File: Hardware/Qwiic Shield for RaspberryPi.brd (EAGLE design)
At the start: 52.3 x 23 mm, 22 parts, among them J1 Qwiic Right Angle, J6 Qwiic Right Angle, J7 Qwiic Right Angle, J8 Qwiic Right Angle, U2 3.3V/600mA

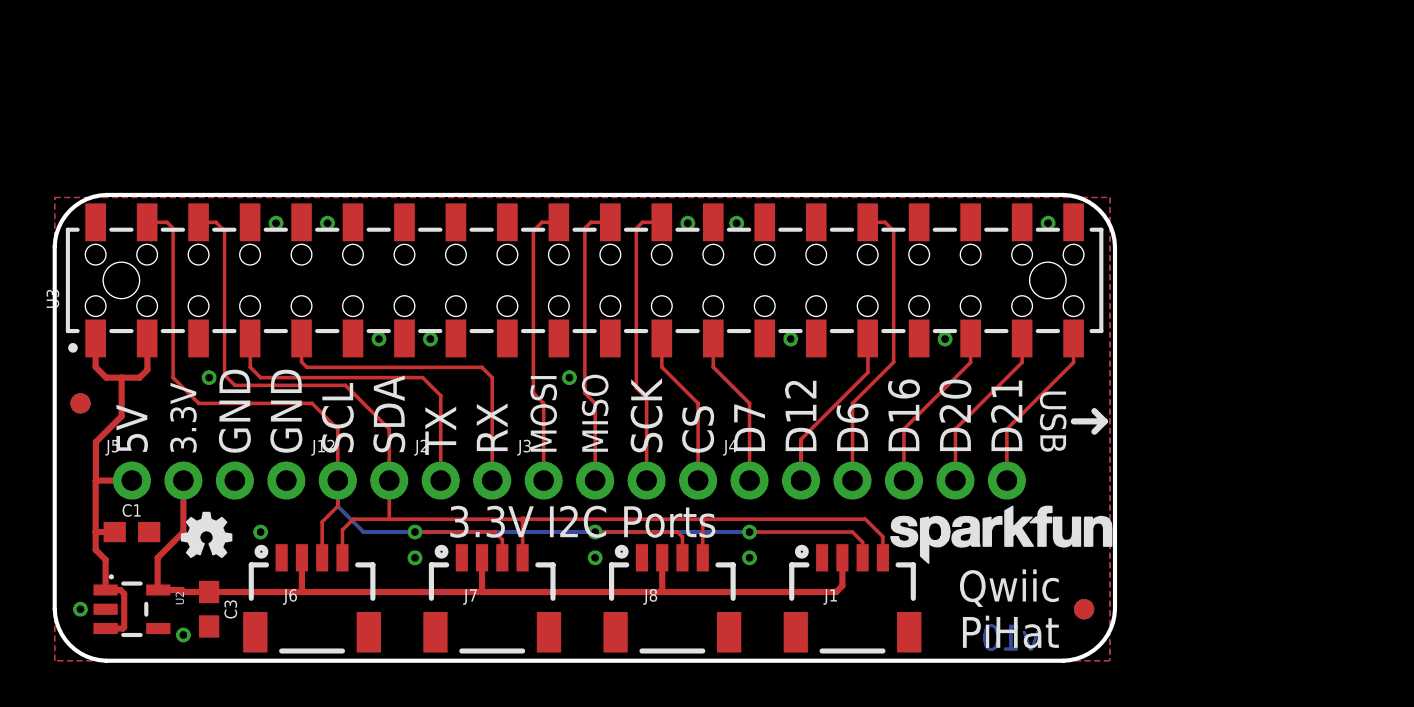
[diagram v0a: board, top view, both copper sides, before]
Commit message: v20 Initial Commit
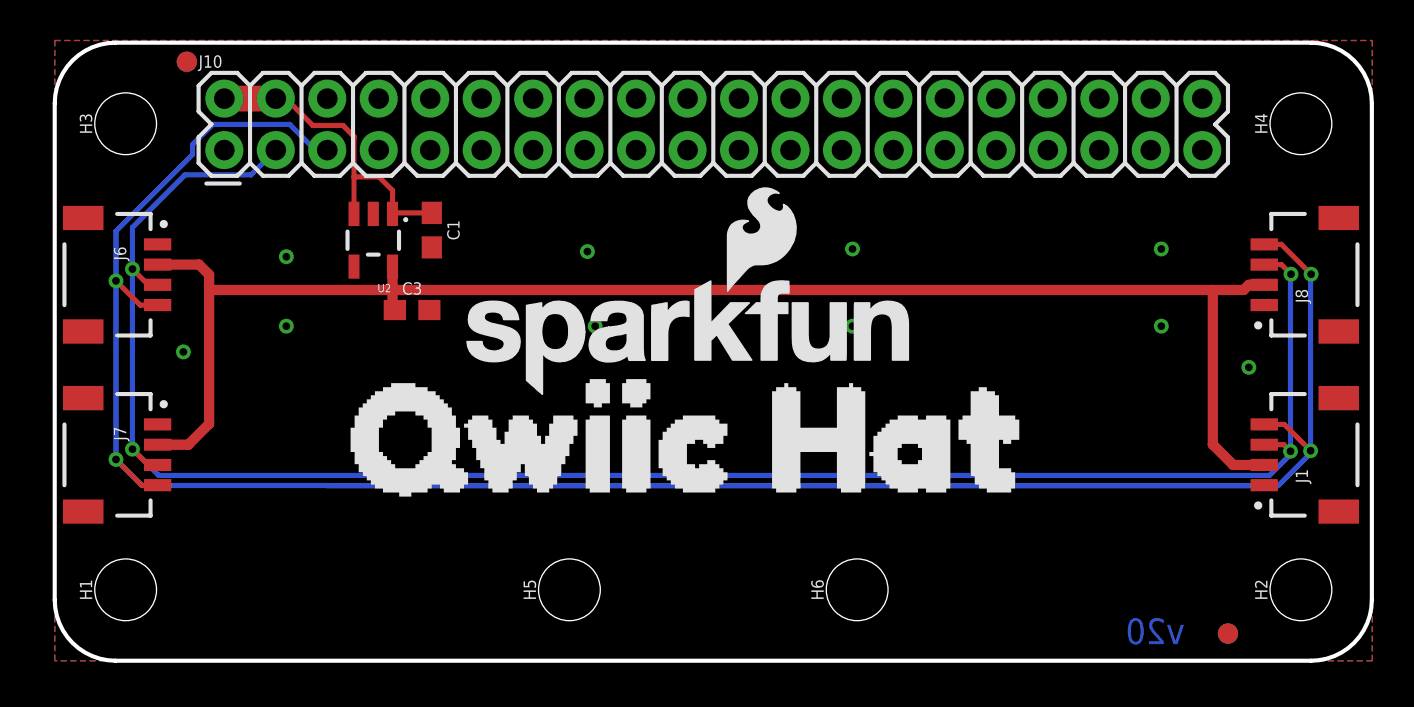
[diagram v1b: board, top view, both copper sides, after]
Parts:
- removed J12, J2: (no value), SparkFun-Connectors:1X02_NO_SILK
- removed J3, J5: (no value), SparkFun-Connectors:1X04_NO_SILK
- removed J4: (no value), SparkFun-Connectors:1X06_NO_SILK
- removed LOGO1: OSHW-LOGOMINI, SparkFun-Aesthetics:OSHW-LOGO-MINI
- removed U$2: SFE_LOGO_NAME.1_INCH, SparkFun-Aesthetics:SFE_LOGO_NAME_.1
- removed U3: (no value), SparkFun-Connectors:RASPBERRY_PI_SHIELD_BOTTOM_ENTRY_NOHOLES
- added H1, H2, H3, H4, H5, H6: STAND-OFFTIGHT, SparkFun-Hardware:STAND-OFF-TIGHT
- added J10: RASPBERRYPI-40-PIN-GPIO_PTH_NO_SHROUD, SparkFun-Connectors:2X20
- added LOGO3: SFE_LOGO_NAME_FLAME.2_INCH, SparkFun-Aesthetics:SFE_LOGO_NAME_FLAME_.2
- J1, J6, J7, J8: device SparkFun-Connectors:1X04_1MM_RA -> SparkFun-Connectors:JST04_1MM_RA
- U$1: value SFE_LOGO_FLAME.1_INCH -> (none); device SparkFun-Aesthetics:SFE_LOGO_FLAME_.1 -> Qwiic Hat:QWIIC_HAT0
- moved J8 32.4 mm to (59.7, 19.1), turned to 90 degrees
- moved U2 21.8 mm to (15.7, 20.8), turned to 180 degrees
- moved C1 21.0 mm to (18.6, 21.2), turned to 270 degrees
- moved J1 20.9 mm to (59.7, 10.2), turned to 90 degrees
- moved C3 17.8 mm to (17.6, 17.3), turned to 0 degrees
- moved FD1 17.7 mm to (6.52, 29.6)
- moved FD4 17.7 mm to (6.52, 29.6)
- moved J7 17.3 mm to (5.08, 10.2), turned to 270 degrees
- moved J6 15.9 mm to (5.08, 19.1), turned to 270 degrees
- moved U$1 8.05 mm to (10.0, 11.0), flipped to the top
- moved FD2 7.20 mm to (57.9, 1.34)
- moved FD3 7.20 mm to (57.9, 1.34)
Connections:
- removed net CS: J3.4, U3.24
- removed net D7: J4.1, U3.26
- new net N$1: J10.17
- new net N$2: J10.1
- net 3.3V: no longer J5.2
- net 5V: now also J10.2, J10.4; no longer J5.1, U3.2, U3.4
- net D12: now also J10.32; no longer J4.2, U3.32
- net D13: now also J10.33; no longer U3.33
- net D16: now also J10.36; no longer J4.4, U3.36
- net D17: now also J10.11; no longer U3.11
- net D18: now also J10.12; no longer U3.12
- net D19: now also J10.35; no longer U3.35
- net D20: now also J10.38; no longer J4.5, U3.38
- net D21: now also J10.40; no longer J4.6, U3.40
- net D22: now also J10.15; no longer U3.15
- net D23: now also J10.16; no longer U3.16
- net D24: now also J10.18; no longer U3.18
- net D25: now also J10.22; no longer U3.22
- net D26: now also J10.37; no longer U3.37
- net D27: now also J10.13; no longer U3.13
- net D4: now also J10.7; no longer U3.7
- net D5: now also J10.29; no longer U3.29
- net D6: now also J10.31; no longer J4.3, U3.31
- net GND: now also J10.14, J10.20, J10.25, J10.30, J10.34, J10.39, J10.6, J10.9; no longer J5.3, J5.4, U3.14, U3.20, U3.25, U3.30, U3.34, U3.39, U3.6, U3.9
- net ID_SCL: now also J10.28; no longer U3.28
- net ID_SDA: now also J10.27; no longer U3.27
- net MISO: now also J10.21; no longer J3.2, U3.21
- net MOSI: now also J10.19; no longer J3.1, U3.19
- net RX: now also J10.10; no longer J2.2, U3.10
- net SCK: now also J10.23; no longer J3.3, U3.23
- net SCL: now also J10.5; no longer J12.2, U3.5
- net SDA: now also J10.3; no longer J12.1, U3.3
- net TX: now also J10.8; no longer J2.1, U3.8
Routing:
- net SCL: track 55.7 -> 104.6 mm, vias 0 -> 4
- net 3.3V: track 46.3 -> 78.1 mm
- net SDA: track 64.1 -> 92.7 mm, vias 3 -> 4
- net RX: track 16.0 -> 0.00 mm
- net TX: track 15.6 -> 0.00 mm
- net D6: track 14.6 -> 0.00 mm
- net MISO: track 14.0 -> 0.00 mm
- net SCK: track 14.0 -> 0.00 mm
- net MOSI: track 14.0 -> 0.00 mm
- net D12: track 8.39 -> 0.00 mm
- net D16: track 8.38 -> 0.00 mm
- net D21: track 8.38 -> 0.00 mm
- net D20: track 8.38 -> 0.00 mm
- net D7: track 7.76 -> 0.00 mm
- net CS: track 7.76 -> 0.00 mm
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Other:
- board size 52.3 x 23 mm -> 65 x 30.5 mm
- board text added: "A. England and Elias Santistevan"
- board text added: "Units in MM"
- board text added: "v20"
- board text removed: "3.3V"
- board text removed: "3.3V I2C Ports"
- board text removed: "5V"
- board text removed: "A. England"
- board text removed: "CS"
- board text removed: "D12"
- board text removed: "D16"
- board text removed: "D20"
- board text removed: "D21"
- board text removed: "D6"
- board text removed: "D7"
- board text removed: "GND"
- board text removed: "MISO"
- board text removed: "MOSI"
- board text removed: "Qwiic PiHat"
- board text removed: "RX"
- board text removed: "SCK"
- board text removed: "SCL"
- board text removed: "SDA"
- board text removed: "TX"
- board text removed: "USB"
- board text removed: "v10"
